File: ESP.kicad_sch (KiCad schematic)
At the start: 23 parts, among them J9 USB_C_Receptacle_USB2.0_16P, U1 TPS2115ADRBR, U4 ESP32-C6-MINI-1/U, U8 LT1963AEST-3.3#TRPBF

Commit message: more bom stuff
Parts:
- C10, C11, C13, C7: footprint Capacitor_SMD:C_0603_1608Metric -> Capacitor_SMD:C_0805_2012Metric
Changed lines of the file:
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@@
 			)
 		)
-		(property "Footprint" "Capacitor_SMD:C_0603_1608Metric"
+		(property "Footprint" "Capacitor_SMD:C_0805_2012Metric"
 			(at 70.8152 92.71 0)
 			(effects
@@
 			)
 		)
-		(property "Footprint" "Capacitor_SMD:C_0603_1608Metric"
+		(property "Footprint" "Capacitor_SMD:C_0805_2012Metric"
 			(at 68.8848 151.13 0)
 			(effects
@@
 			)
 		)
-		(property "Footprint" "Capacitor_SMD:C_0603_1608Metric"
+		(property "Footprint" "Capacitor_SMD:C_0805_2012Metric"
 			(at 216.2302 149.225 0)
 			(effects
@@
 			)
 		)
-		(property "Footprint" "Capacitor_SMD:C_0603_1608Metric"
+		(property "Footprint" "Capacitor_SMD:C_0805_2012Metric"
 			(at 41.6052 92.71 0)
 			(effects

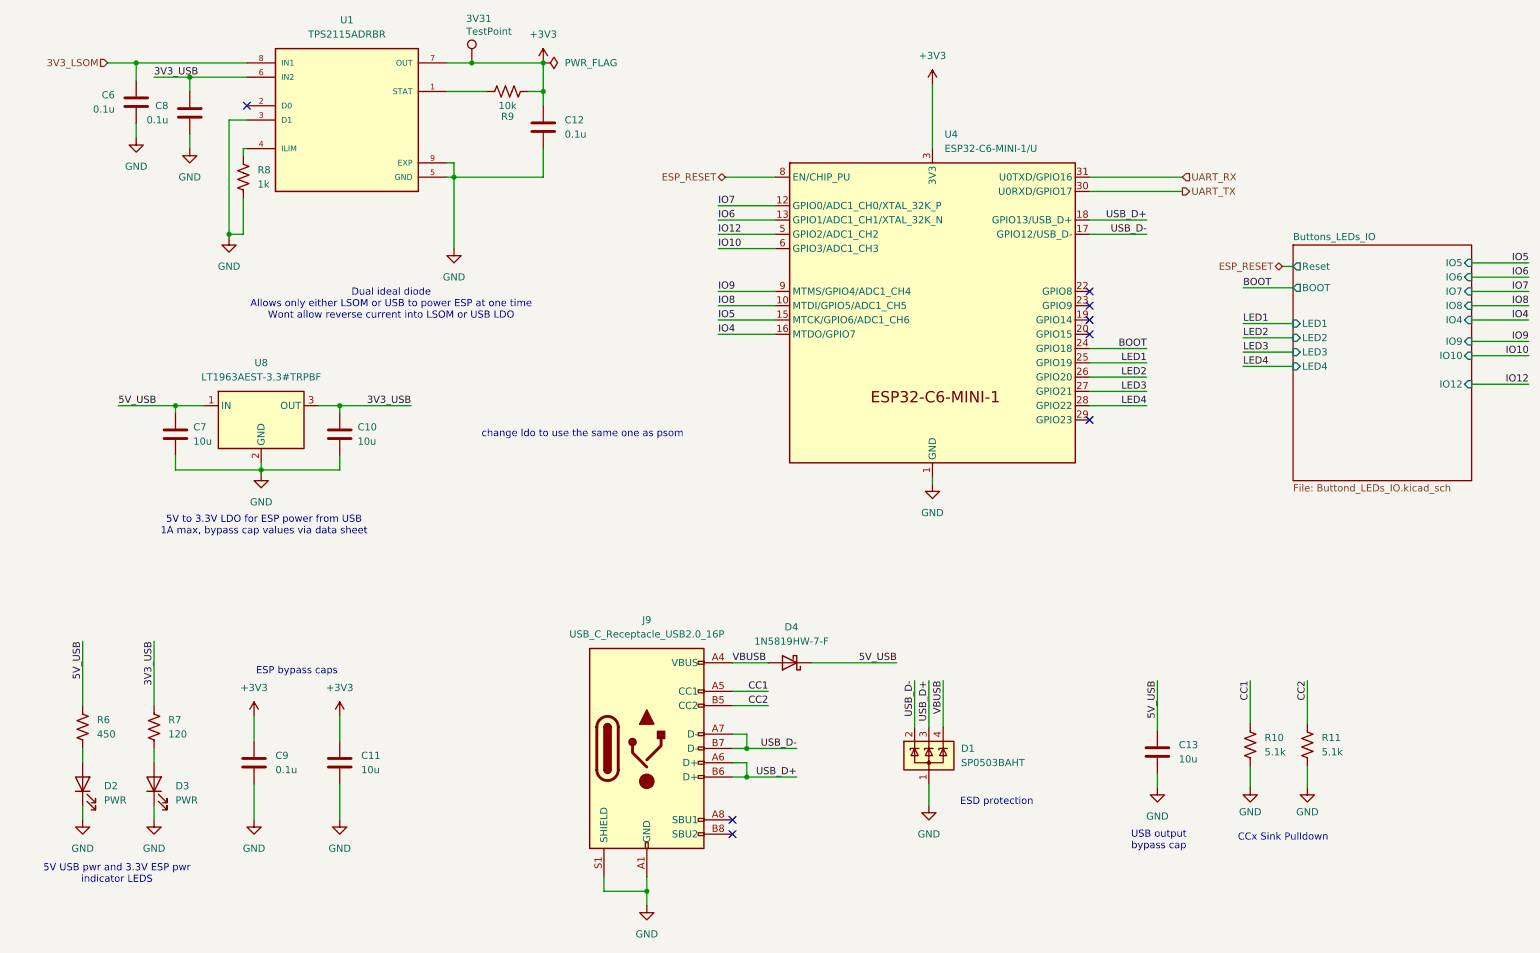
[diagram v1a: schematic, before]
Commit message: start of RevB. BOM for revA
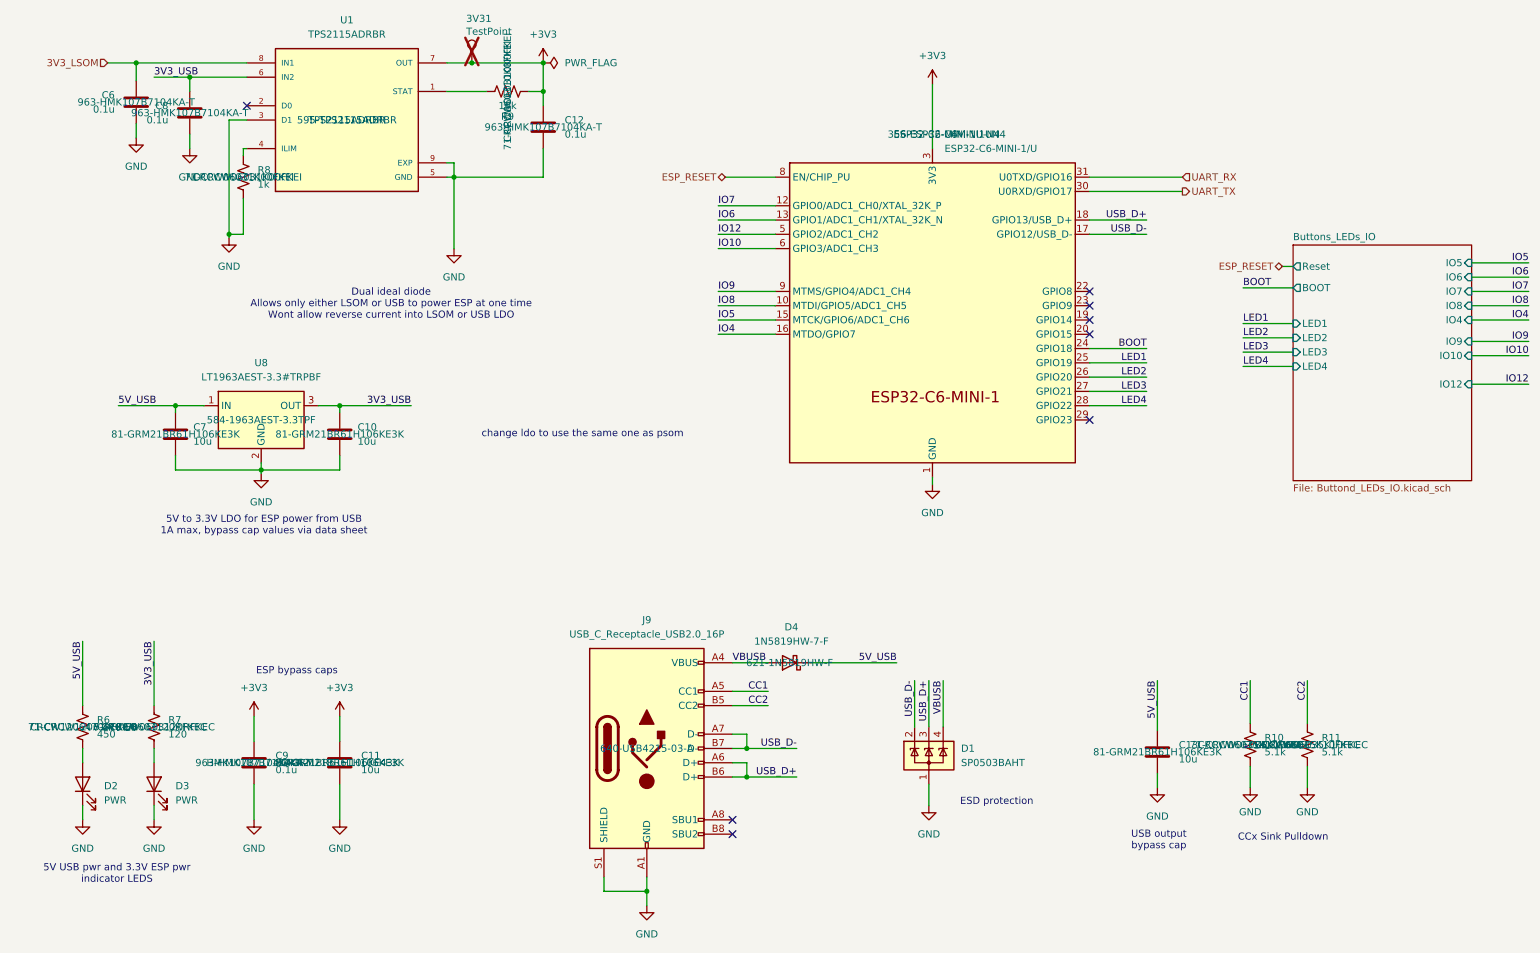
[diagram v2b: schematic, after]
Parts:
- 3V31: now not fitted; now left out of the parts list
- C10, C13: Mouser Part Number (none) -> 81-GRM21BR61H106KE3K; P/N MLAST168BB5106MTNA01 -> GRM21BR61H106KE43K
- C11: Mouser Part Number (none) -> 81-GRM21BR61H106KE3K; P/N (none) -> GRM21BR61H106KE43K
- C12, C6, C8: Mouser Part Number (none) -> 963-HMK107B7104KA-T; P/N UMK107B7104KAHT -> HMK107B7104KA-T
- C7: Mouser Part Number (none) -> 81-GRM21BR61H106KE3K; P/N UMK107B7104KAHT -> GRM21BR61H106KE43K
- C9: Mouser Part Number (none) -> 963-HMK107B7104KA-T; P/N (none) -> HMK107B7104KA-T
- D2, D3: P/N HSML-C191 -> XL-1608UBC-06A
- D4: Mouser Part Number (none) -> 621-1N5819HW-F
- J9: Mouser Part Number (none) -> 640-USB4215-03-A
- R10, R11: Mouser Part Number (none) -> 71-CRCW06035K10FKEC; P/N (none) -> CRCW06035K10FKEC
- R6: Mouser Part Number (none) -> 71-CRCW1206-470-E3; P/N (none) -> CRCW1206470RFKEA
- R7: Mouser Part Number (none) -> 71-CRCW0603120RFKEC; P/N (none) -> CRCW0603120RFKEC
- R8: Mouser Part Number (none) -> 71-CRCW06031K00FKEI; P/N (none) -> CRCW06031K00FKEI
- R9: Mouser Part Number (none) -> 71-CRCW060310K0FKEI; P/N (none) -> CRCW060310K0FKEI
- U1: Mouser Part Number (none) -> 595-TPS2115ADRBR; P/N (none) -> TPS2115ADRBR
- U4: Mouser Part Number (none) -> 356-ESP32-C6MINI1UN4; P/N (none) -> ESP32-C6-MINI-1U-N4
- U8: Mouser Part Number (none) -> 584-1963AEST-3.3TPF; P/N LT1963AEST-3.3#TRPBF -> LT1963AEST-3.3#TRPBF
